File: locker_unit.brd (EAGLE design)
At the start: 58 x 52 mm, 30 parts, among them IC2 7805T, J1 RJ11, J2 RJ11, Q2 8 MHz, Q4 BC547, U1 PIC16F1705-X/PDIP

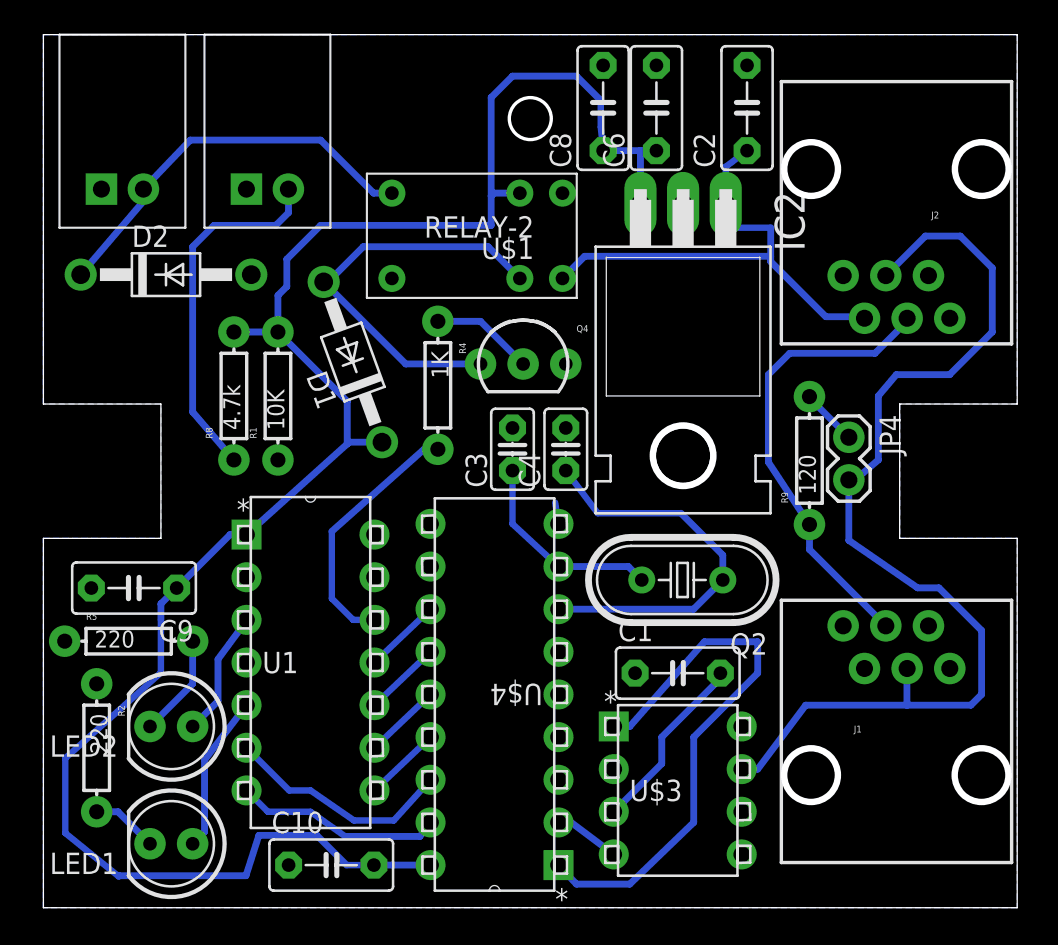
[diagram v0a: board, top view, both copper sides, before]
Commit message: Edit whole layout, add external LED header. Should be the final version.
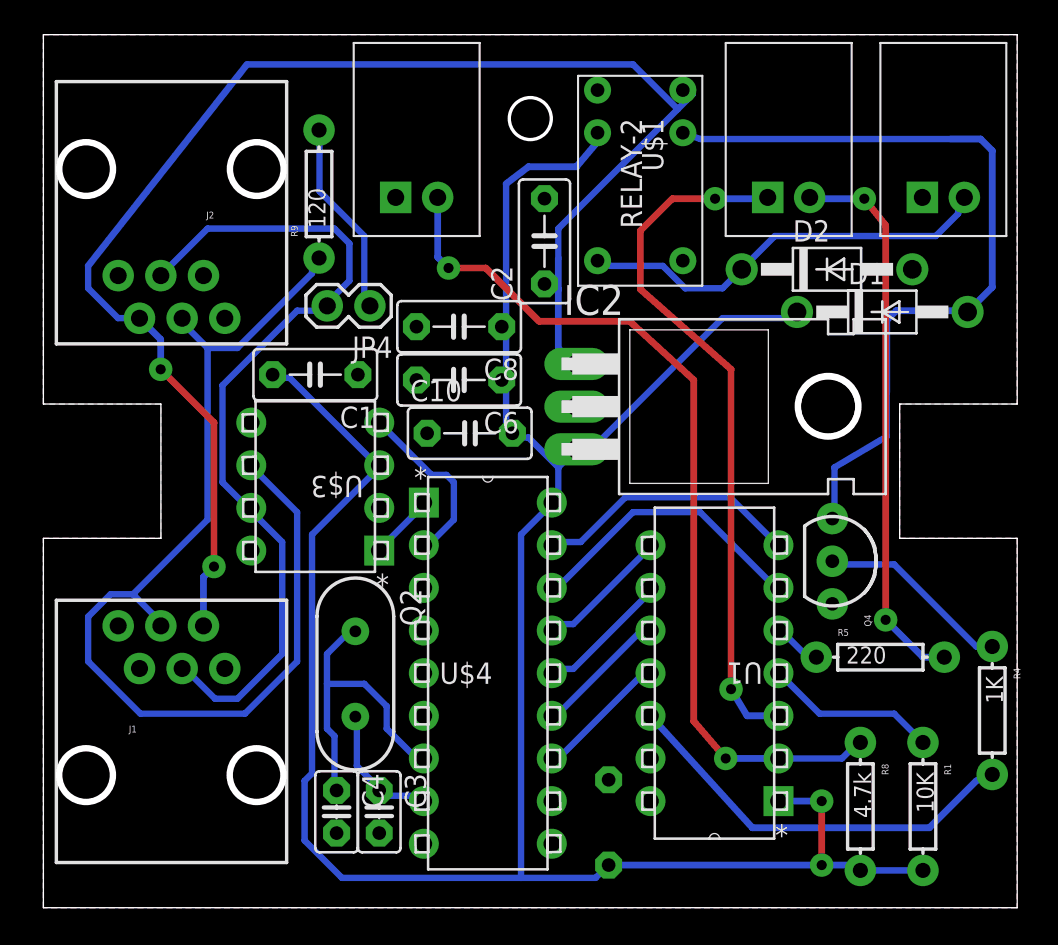
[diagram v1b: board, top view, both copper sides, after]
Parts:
- removed LED1: RED, SparkFun-LED:LED5MM
- removed LED2: GREEN, SparkFun-LED:LED5MM
- removed R2: 220, SparkFun-Passives:AXIAL-0.3
- added X3: (no value), Locker-custom:KK-156-2
- Q2: device crystal:HC49U70 -> SparkFun-FreqCtrl:HC49US
- moved X2 48.9 mm to (49.9, 40.0)
- moved R1 45.5 mm to (52.4, 6.03), turned to 270 degrees
- moved R5 44.8 mm to (49.8, 14.9)
- moved R8 44.6 mm to (48.7, 6.03), turned to 270 degrees
- moved J1 43.2 mm to (7.63, 7.90)
- moved J2 43.2 mm to (7.63, 44.0)
- moved D2 39.4 mm to (46.7, 38.0)
- moved U$3 38.9 mm to (12.4, 28.9), turned to 180 degrees
- moved R4 38.3 mm to (56.5, 11.7)
- moved R9 33.2 mm to (16.4, 42.5)
- moved D1 31.7 mm to (50.0, 35.5), turned to 0 degrees
- moved C9 31.5 mm to (33.7, 5.08), flipped to the bottom, turned to 90 degrees
- moved JP4 29.6 mm to (19.4, 35.8), turned to 180 degrees
- moved C1 28.0 mm to (16.2, 31.8), turned to 180 degrees
- moved C10 27.0 mm to (25.4, 28.3)
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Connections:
- removed net N$7: LED2.K, R5.P$2
- net GND: no longer R2.P$1, R5.P$1
- net N$12: now also X3.2; no longer LED2.A
- net N$2: now also R5.P$1; no longer LED1.A
- net N$5: now also R5.P$2, X3.1; no longer LED1.K, R2.P$2
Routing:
- net 12V: track 32.2 -> 89.1 mm, vias 0 -> 2
- net CANL: track 27.3 -> 64.6 mm
- net N$12: track 7.54 -> 41.8 mm, vias 0 -> 2
- net N$16: track 21.6 -> 53.4 mm, vias 0 -> 2
- net N$5: track 3.96 -> 33.7 mm, vias 0 -> 2
- net TXCAN: track 33.2 -> 3.96 mm
- net 5V: track 124.9 -> 148.3 mm, vias 0 -> 2
- net N$3: track 24.7 -> 47.7 mm
- net CANH: track 62.3 -> 50.7 mm
- net N$6: track 0.00 -> 10.3 mm
- net LOCK_CTRL: track 15.2 -> 24.5 mm
- net N$17: track 3.39 -> 11.8 mm
- net RXCAN: track 3.93 -> 10.9 mm
- net N$2: track 9.40 -> 3.11 mm
- net N$7: track 6.13 -> 0.00 mm
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- added copper zone on layer 1, net GND
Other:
- outline, holes or cut-outs redrawn
